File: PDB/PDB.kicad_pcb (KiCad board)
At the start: 2 copper layers, 111.8 x 88.1 mm, 45 parts, among them J1 Conn_01x02, J2 Conn_01x04, Q1 S8050, Sw1 D-SWITCH_MR5-111-C5N-BB, Y1 12MHz

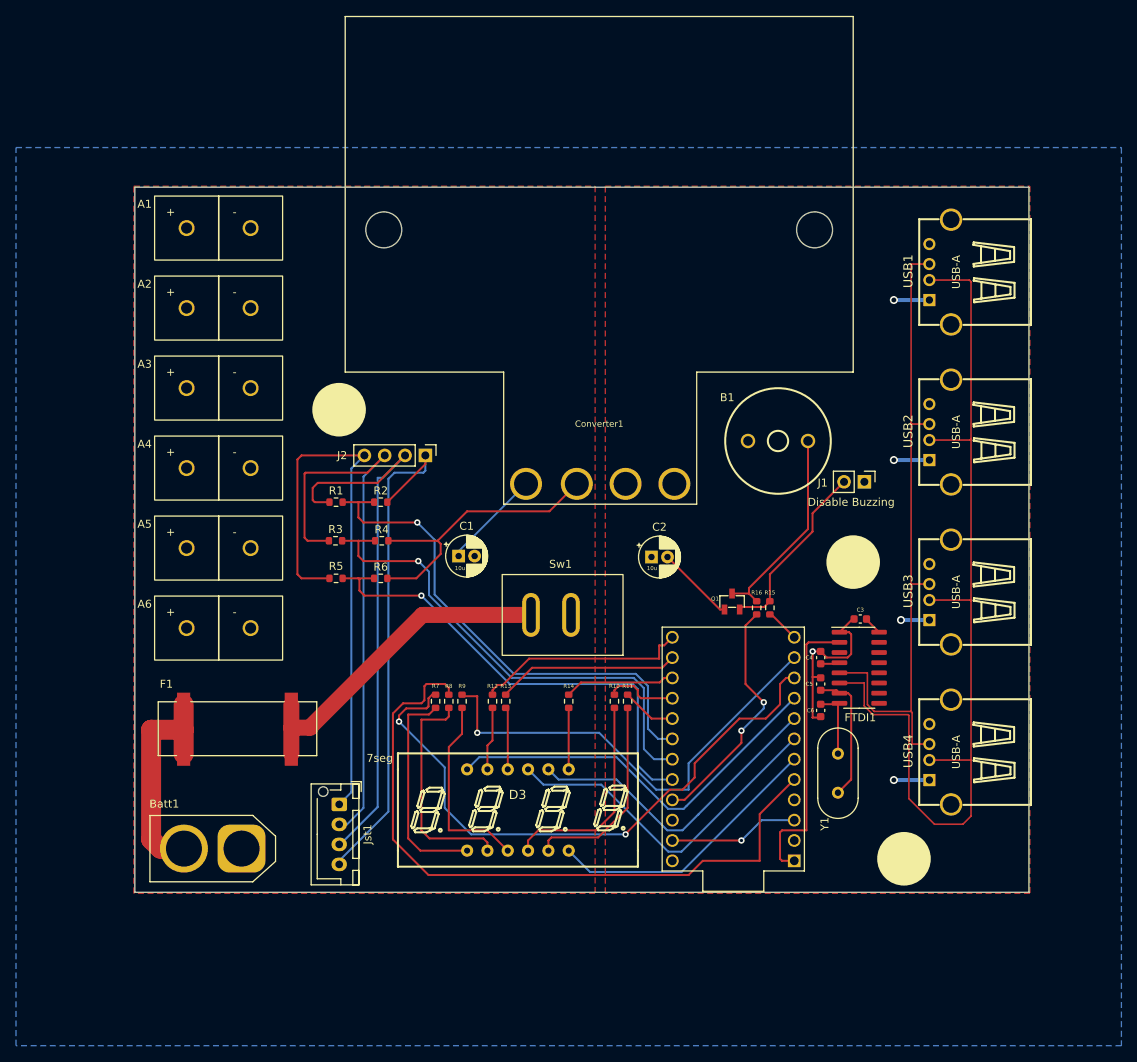
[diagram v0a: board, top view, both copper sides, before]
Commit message: Finished board layout?
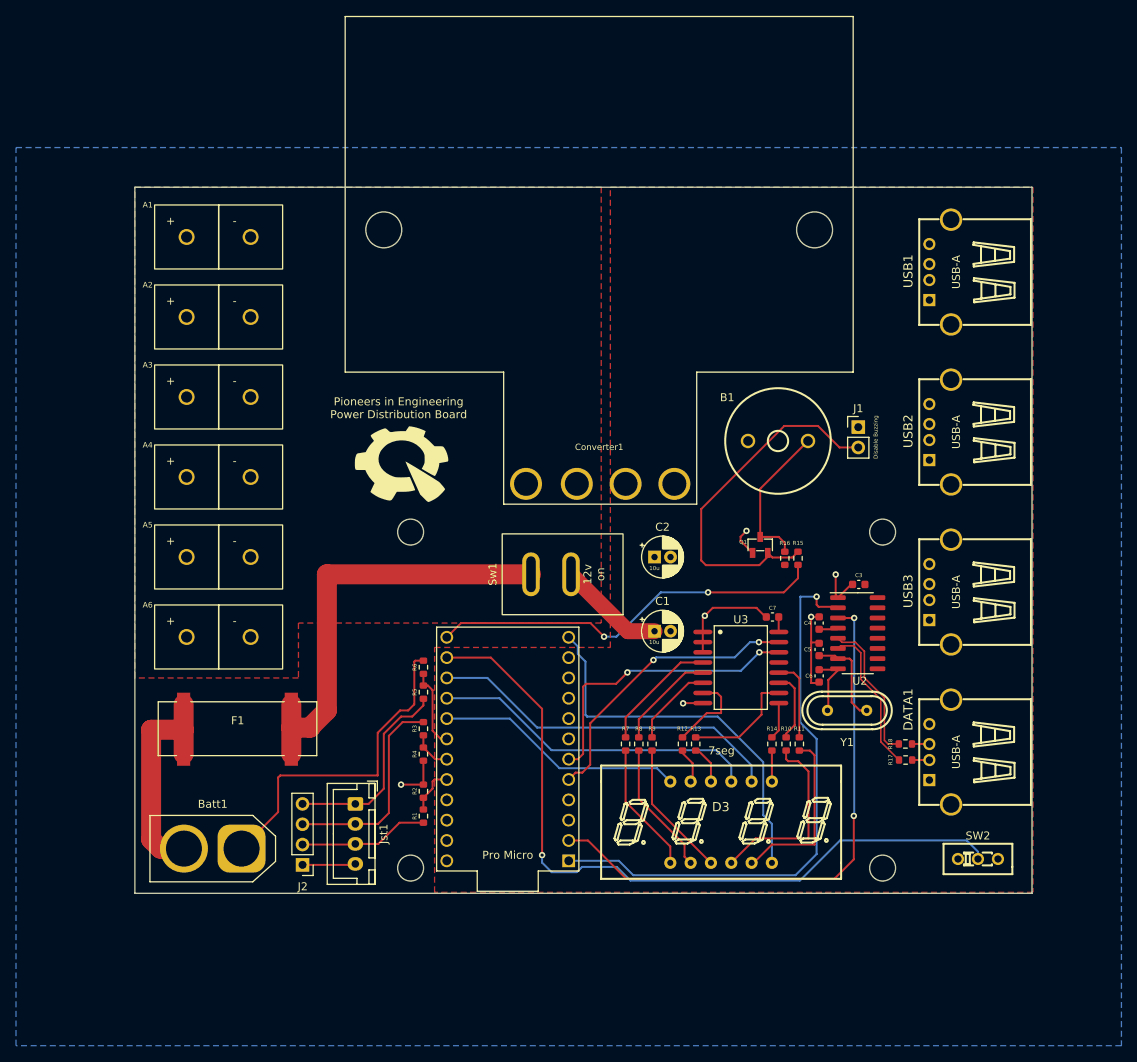
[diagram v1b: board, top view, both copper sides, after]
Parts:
- added ?: , , F.Cu at (92.0, 102.0)
- added ?: , , F.Cu at (151.0, 102.0)
- added ?: , , F.Cu at (93.5, 53.2)
- added ?: , , F.Cu at (151.0, 60.0)
- added C7: 0.1u, Capacitor_SMD:C_0603_1608Metric, F.Cu at (137.2, 70.6)
- added G***: LOGO, PiE_Footprints:PiE Logo, F.Cu at (91.0, 51.5)
- added R17: 22, Resistor_SMD:R_0603_1608Metric, F.Cu at (153.9, 88.5)
- added R18: 22, Resistor_SMD:R_0603_1608Metric, F.Cu at (153.8, 86.5)
- added SW2: SW_SPDT, PiE_Footprints:DEALON SS-12D01-G3, F.Cu at (162.9, 100.9)
- added U3: PCF8574, PiE_Footprints:PCF8574T, F.Cu at (133.3, 76.9)
- Batt1: footprint PiE_Footprints:XT60_F -> PiE_Footprints:AMASS_XT60-M_1x02_P7.20mm_Vertical
- J1: footprint Connector_PinHeader_2.54mm:PinHeader_1x02_P2.54mm_Vertical -> PiE_Footprints:PinHeader_1x02_P2.54mm_Vertical
- J2: footprint Connector_PinHeader_2.54mm:PinHeader_1x04_P2.54mm_Vertical -> PiE_Footprints:PinHeader_1x04_P2.54mm_Vertical
- Jst1: footprint PiE_Footprints:JST_XH_B4B-XH-AM_1x04_P2.50mm_Vertical -> PiE_Footprints:JST_XH_B4B-XH-A_1x04_P2.50mm_Vertical
- Y1: footprint Crystal:Crystal_HC49-U_Vertical -> PiE_Footprints:JYJE S1C12000VWFAC
- moved J2 53.4 mm to (78.5, 101.6), turned to 180 degrees
- moved R1 40.7 mm to (93.6, 95.5), turned to 90 degrees
- moved R2 36.5 mm to (93.6, 92.4), turned to 90 degrees
- moved Pro1 28.2 mm to (104.1, 87.1)
- moved R4 27.2 mm to (93.6, 87.8), turned to 90 degrees
- moved C1 26.2 mm to (122.5, 72.4)
- moved R14 26.0 mm to (137.2, 86.5)
- moved R3 25.9 mm to (93.6, 84.6), turned to -90 degrees
- moved D3 25.4 mm to (130.8, 96.3)
- moved R13 24.3 mm to (127.6, 86.5)
- moved R9 24.3 mm to (122.2, 86.5)
- moved R12 24.3 mm to (126.0, 86.5)
- moved R7 24.3 mm to (118.9, 86.5)
- moved R8 24.3 mm to (120.5, 86.5)
- moved R10 22.1 mm to (138.9, 86.5)
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- renumbered USB4 to DATA1, FTDI1 to U2
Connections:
- DATA1 pad 2: /D- -> Net-(DATA1-Pad2)
- DATA1 pad 3: /D+ -> Net-(DATA1-Pad3)
- Pro1 pad 10: /E -> unconnected-(Pro1-Pad10)
- Pro1 pad 11: /DP -> unconnected-(Pro1-Pad11)
- Pro1 pad 12: /Buzzer -> /Dig4
- Pro1 pad 13: /A -> /Buzzer
- Pro1 pad 14: /F -> /toggle
- Pro1 pad 15: /B -> /Dig3
- Pro1 pad 16: /C -> /Dig2
- Pro1 pad 17: /G -> /Dig1
- Pro1 pad 18: /Cell1_s -> /Cell1+2+3_s
- Pro1 pad 2: /toggle -> /Rx
- Pro1 pad 20: /Cell1+2+3_s -> /Cell1_s
- Pro1 pad 5: /D -> /SDA
- Pro1 pad 6: /Dig4 -> /SCL
- Pro1 pad 7: /Dig2 -> unconnected-(Pro1-Pad7)
- Pro1 pad 8: /Dig3 -> unconnected-(Pro1-Pad8)
- Pro1 pad 9: /Dig1 -> unconnected-(Pro1-Pad9)
- U2 pad 3: unconnected-(FTDI1-Pad3) -> /Rx
- USB1 pad 2: /D- -> unconnected-(USB1-Pad2)
- USB1 pad 3: /D+ -> unconnected-(USB1-Pad3)
- USB2 pad 2: /D- -> unconnected-(USB2-Pad2)
- USB2 pad 3: /D+ -> unconnected-(USB2-Pad3)
- USB3 pad 2: /D- -> unconnected-(USB3-Pad2)
- USB3 pad 3: /D+ -> unconnected-(USB3-Pad3)
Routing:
- net /D-: track 119.8 -> 18.7 mm
- net /toggle: track 0.00 -> 93.3 mm, vias 0 -> 1
- net /D: track 86.7 -> 12.7 mm
- net /Rx: track 0.00 -> 70.8 mm, vias 0 -> 2
- net /D+: track 82.4 -> 18.1 mm
- net /E: track 75.9 -> 15.0 mm, vias 2 -> 0
- net GND: track 150.0 -> 89.8 mm, vias 2 -> 6
- net /Cell1_s: track 63.7 -> 5.85 mm, vias 1 -> 0
- net /Cell1+2_s: track 62.0 -> 5.05 mm, vias 1 -> 0
- net /Cell1: track 69.4 -> 16.2 mm
- net /Cell1+2+3_s: track 60.0 -> 10.1 mm, vias 1 -> 0
- net /5v: track 49.5 -> 1.96 mm, vias 6 -> 0
- net /DP: track 57.9 -> 10.5 mm, vias 1 -> 0
- net /Cell1+2+3: track 72.1 -> 25.1 mm
- net /Buzzer: track 4.23 -> 50.0 mm, vias 0 -> 2
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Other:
- board size 111.8 x 88.1 mm -> 112.1 x 88.3 mm
- board text added: "1"
- board text added: "1+2"
- board text added: "1+2+3"
- board text added: "12v"
- board text added: "12v on"
- board text added: "5v"
- board text added: "Copyright (c) 2023, Pioneers in Engineering All rights reserved. Design by: Justin H This design is open source hardware. For more information, visit github.com/pioneers/PiElectrical"
- board text added: "GND"
- board text added: "Pioneers in Engineering Power Distribution Board"
- board text added: "Pro Micro"
